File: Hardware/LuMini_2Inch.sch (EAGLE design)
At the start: 51 parts, among them J1 DOUBLE_LED_PAD, J2 DOUBLE_LED_PAD, J3 DOUBLE_LED_PAD

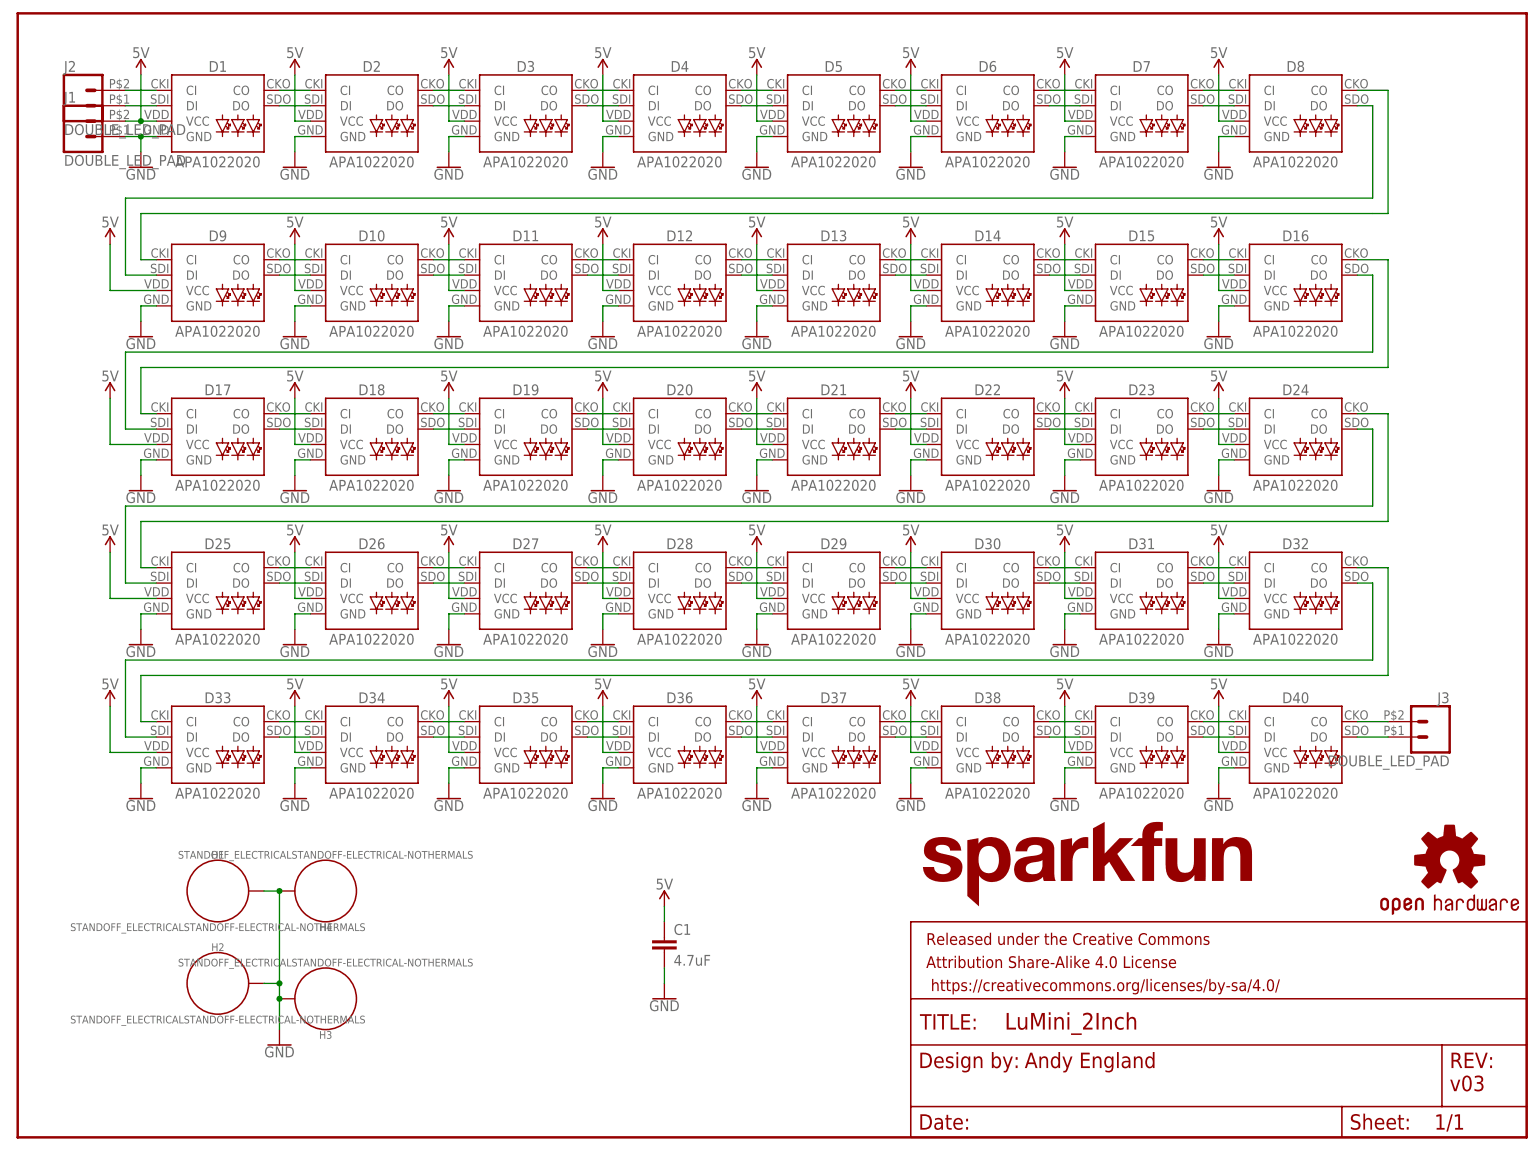
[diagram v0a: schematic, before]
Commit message: post checklist
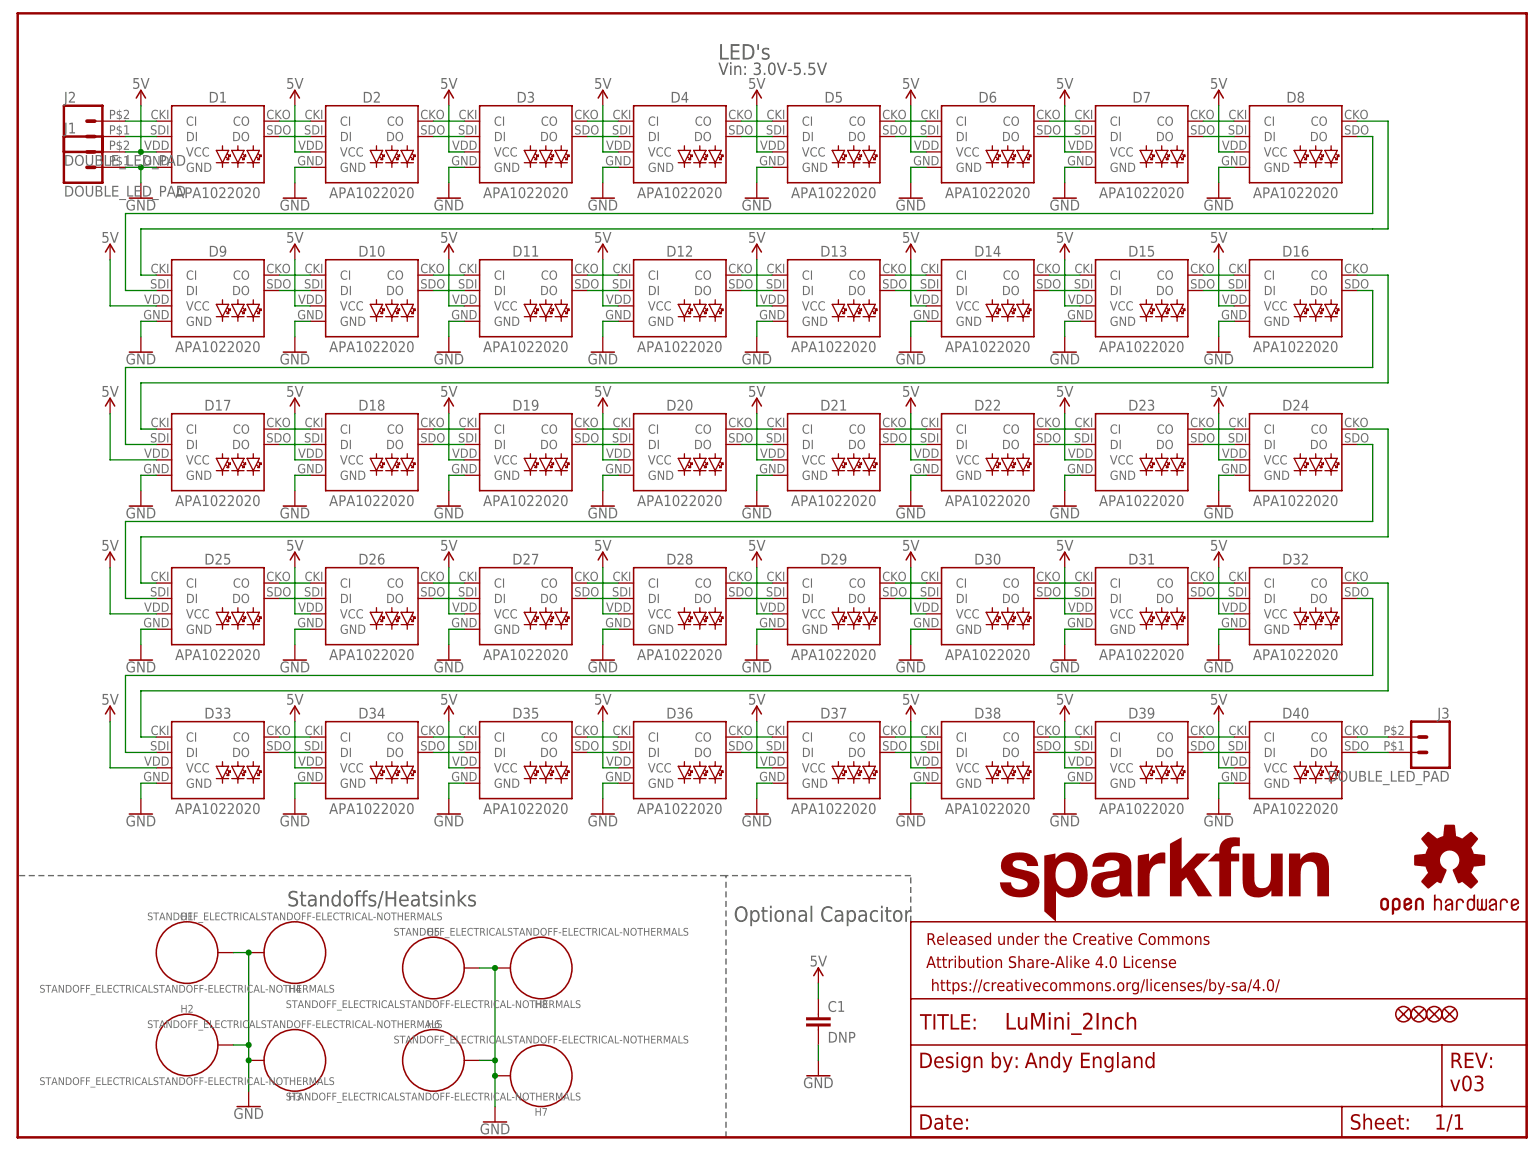
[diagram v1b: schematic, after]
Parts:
- added FD1, FD2, FD3, FD4: FIDUCIALUFIDUCIAL, SparkFun-Aesthetics:FIDUCIALUFIDUCIAL
- added H5, H6, H7, H8: STANDOFF_ELECTRICALSTANDOFF-ELECTRICAL-NOTHERMALS, SparkFun-Hardware:STANDOFF_ELECTRICALSTANDOFF-ELECTRICAL-NOTHERMALS
- C1: value 4.7uF -> DNP; device SparkFun-Capacitors:4.7UF-0603-6.3V-(10%) -> SparkFun-Capacitors:4.7UF-1206-16V-(+80/-20%)
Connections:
- net GND: now also H5.P$1, H6.P$1, H7.P$1, H8.P$1
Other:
- note added: "LED's"
- note added: "Optional Capacitor"
- note added: "Standoffs/Heatsinks"
- note added: "Vin: 3.0V-5.5V"
- moved on the sheet: C1, D1, D10, D11, D12, D13, D14, D15, D16, D17, D18, D19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
